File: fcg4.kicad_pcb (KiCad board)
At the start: 4 copper layers, 34 x 33.5 mm, 99 parts, among them IC1 MP9943AGQ-Z, IC2 MP9943AGQ-Z, J1 USB4105-GF-A-120, J2 SM08B-SRSS-TB, U1 STM32G473CEUx, U10 MAX40200ANS_T, U11 MAX40200ANS_T, U2 ICM-42688-P, U4 AP2112K-3.3TRG1, U5 AP2112K-1.8TRG1, Y1 ECS-240-6-37B-7KM-TR

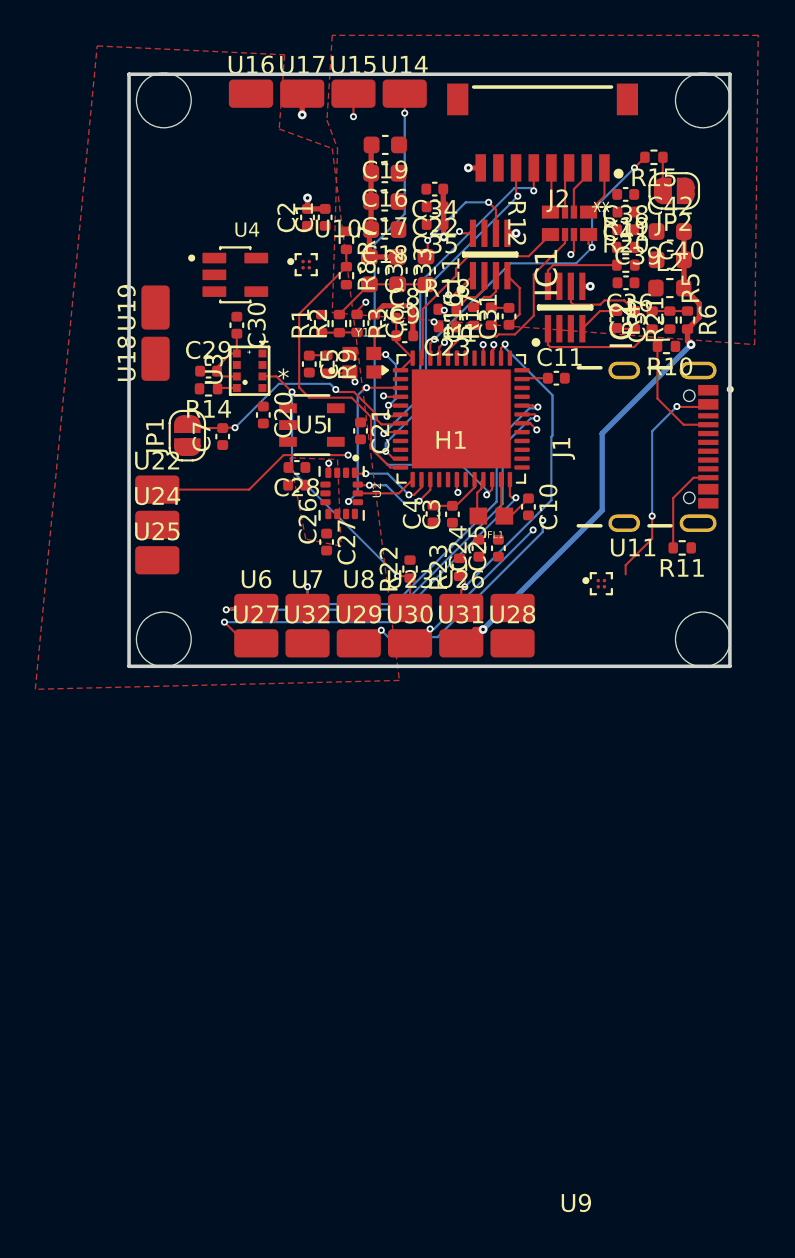
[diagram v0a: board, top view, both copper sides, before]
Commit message: routing...
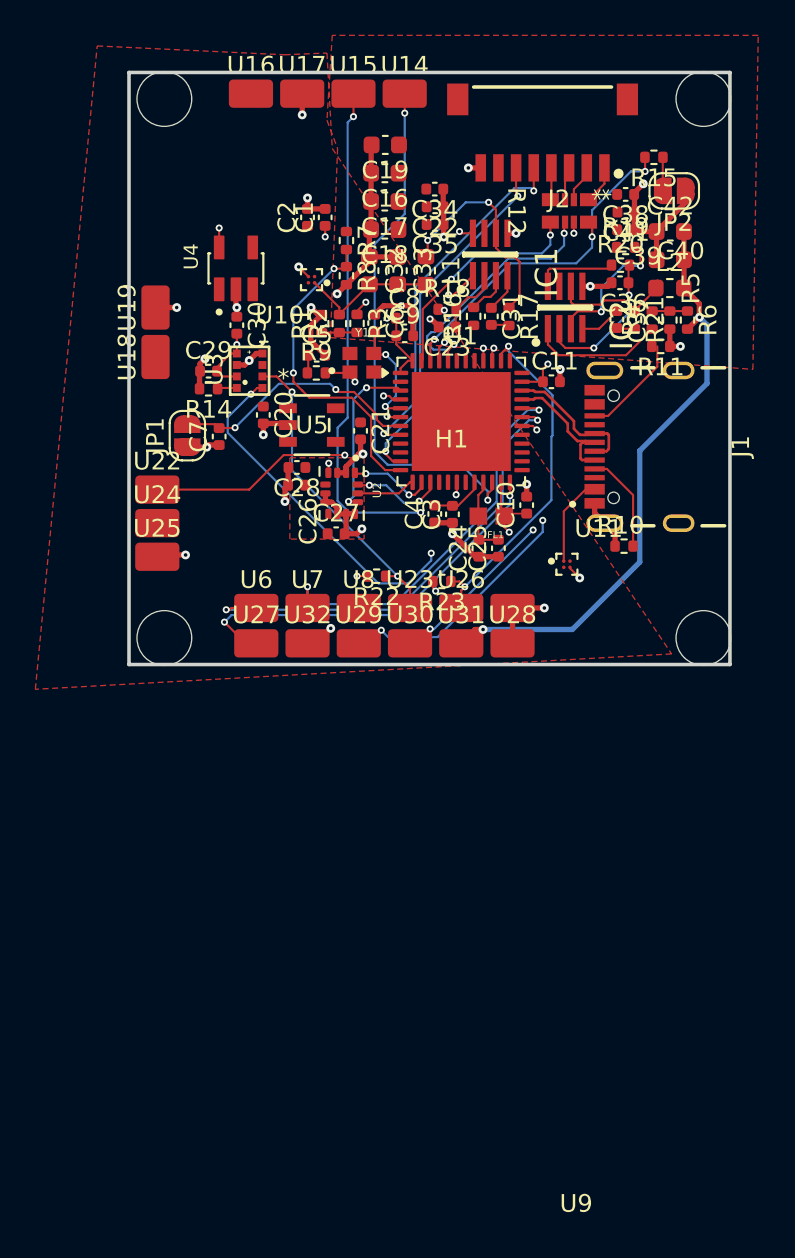
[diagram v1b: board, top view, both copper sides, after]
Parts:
- moved R10 11.6 mm to (28.0, 27.2), turned to 0 degrees
- moved R11 11.5 mm to (30.1, 15.9)
- moved J1 3.08 mm to (31.1, 21.6), turned to 90 degrees
- moved U11 2.24 mm to (24.8, 28.2)
- moved R22 1.93 mm to (14.0, 28.9), turned to 180 degrees
- moved R23 1.28 mm to (17.7, 29.2), turned to 180 degrees
- moved R17 1.00 mm to (21.5, 14.2), turned to -90 degrees
- moved C31 1.00 mm to (20.5, 14.2), turned to -90 degrees
- moved U10 0.90 mm to (10.3, 12.1), turned to 180 degrees
- moved R9 0.77 mm to (10.6, 17.4), turned to 0 degrees
- moved C27 0.72 mm to (11.7, 26.5), turned to 0 degrees
- moved R12 0.70 mm to (24.9, 8.23)
- moved C5 0.65 mm to (10.6, 16.4), turned to 0 degrees
- moved U4 0.37 mm to (6.05, 11.5), turned to 90 degrees
- moved C11 0.34 mm to (23.9, 17.9)
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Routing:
- net GND: track 19.6 -> 75.9 mm, vias 8 -> 29
- net I2C1_SCL: track 19.8 -> 42.1 mm, vias 2 -> 4
- net /Power/BIAS_SUPPLY_9V: track 0.00 -> 8.40 mm, vias 0 -> 2
- net /MCU/USB_DIFF+: track 0.00 -> 7.92 mm
- net /MCU/USB_DIFF-: track 0.00 -> 7.91 mm
- net /Power/EN/SYNC_9V: track 0.00 -> 7.76 mm, vias 0 -> 2
- net 5V_USB: track 12.5 -> 5.08 mm, vias 2 -> 0
- net VDD_MCU: track 13.1 -> 18.4 mm, vias 0 -> 8
- net /Power/LC_5V5: track 7.23 -> 12.6 mm
- net 9V_BEC: track 29.7 -> 33.8 mm
- net MOTOR3: track 11.4 -> 14.5 mm, vias 0 -> 2
- net RX3: track 59.7 -> 56.7 mm, vias 3 -> 4
- net 5V5_BEC: track 5.62 -> 8.00 mm
- net /MCU/VDDA: track 2.24 -> 4.49 mm
- net /Power/LC_9V: track 4.91 -> 6.69 mm
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- added copper zone on In2.Cu, net VDD_MCU

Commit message: routing...
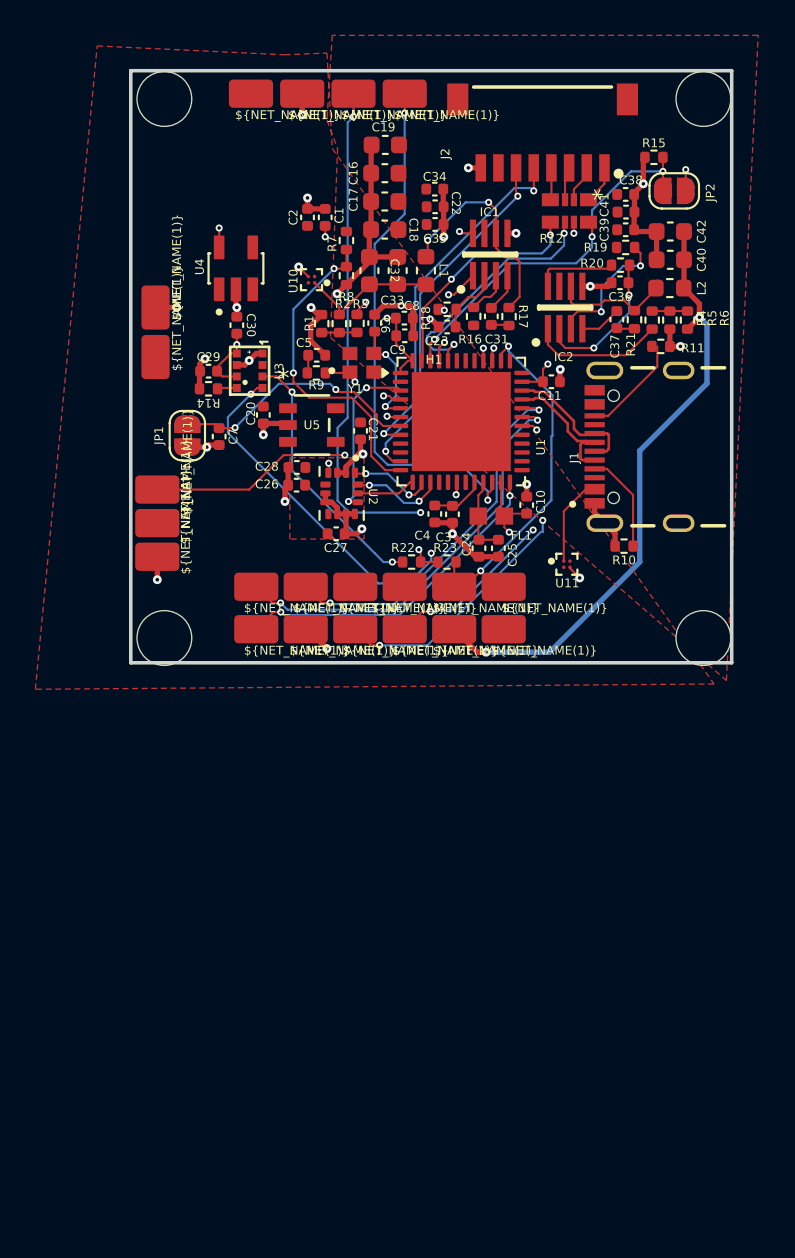
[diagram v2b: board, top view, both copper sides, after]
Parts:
- moved R22 2.14 mm to (16.0, 28.1), turned to 0 degrees
- moved U9 1.30 mm to (21.2, 29.5)
- moved U26 1.26 mm to (18.4, 29.5)
- moved U23 1.24 mm to (15.6, 29.5)
- moved U8 1.22 mm to (12.8, 29.5)
- moved U7 1.20 mm to (10.0, 29.5)
- moved U6 1.20 mm to (7.20, 29.5)
- moved R23 1.14 mm to (18.0, 28.1)
- moved U28 0.94 mm to (21.2, 31.9)
- moved U31 0.89 mm to (18.4, 31.9)
- moved U30 0.85 mm to (15.6, 31.9)
- moved U29 0.82 mm to (12.8, 31.9)
- moved U32 0.81 mm to (10.0, 31.9)
- moved U27 0.80 mm to (7.20, 31.9)
- turned R15 to 0 degrees
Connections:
- JP2 pad 1: GND -> VDD_MCU
- JP2 pad 2: /MCU/BOOT0 -> MOTOR1
- R15 pad 1: /MCU/BOOT0 -> GND
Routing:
- net GND: track 75.9 -> 70.3 mm, vias 29 -> 28
- net RX3: track 56.7 -> 52.9 mm
- net TX1: track 26.6 -> 23.7 mm
- net I2C1_SDA: track 28.8 -> 26.0 mm
- net MOTOR1: track 20.1 -> 22.2 mm
- net /MCU/BOOT0: track 1.90 -> 0.00 mm
- net VDD_MCU: track 18.4 -> 20.1 mm
- net RX1: track 22.6 -> 21.2 mm
- net I2C1_SCL: track 42.1 -> 43.5 mm
- net 9V_BEC: track 33.8 -> 34.9 mm
